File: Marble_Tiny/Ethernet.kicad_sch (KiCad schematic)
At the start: 38 parts, among them J3 BELFUSE_0826-1G1T-43-F, Q1 XTAL_25MHZ_EPSON_TSX-3225_25.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, U7 RTL8211F-CG

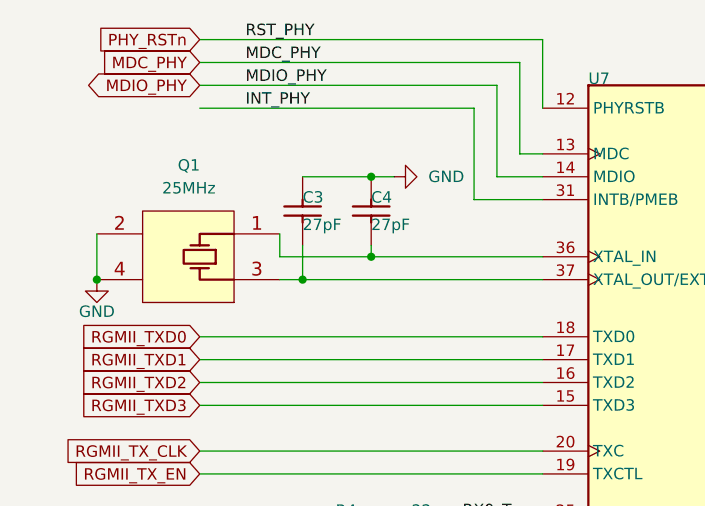
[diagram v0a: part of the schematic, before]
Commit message: components placement and PCB routing
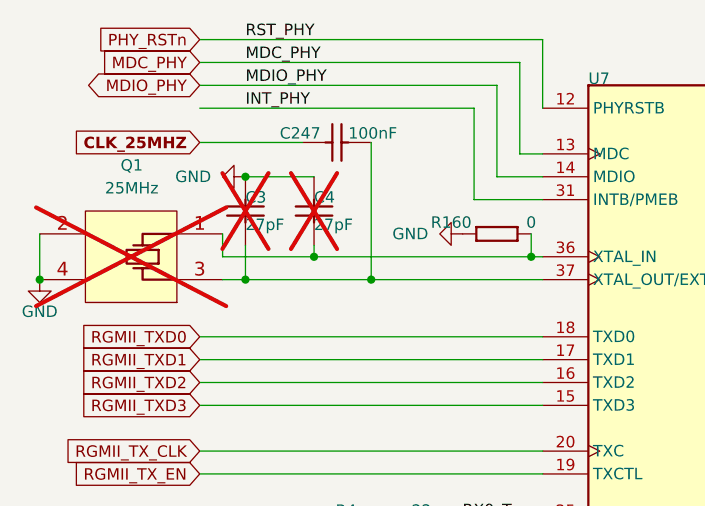
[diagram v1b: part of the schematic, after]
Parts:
- added C247: CC0402_100NF_50V_10%_X7R, Capacitors SMD:CAPC1005X55N, symbol Capacitors SMD:CC0402_100NF_50V_10%_X7R
- added R160: R0402_0R_JUMPER, RESC1005X40N, symbol Resistors_SMD:R0402_0R_JUMPER
- C3, C4, Q1: now not fitted
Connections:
- net GND: now also R160.1
- net at C4.1, Q1.1 (X), U7.36 (XTAL_IN): now also R160.2
- net at C3.1, Q1.3 (X), U7.37 (XTAL_OUT/EXT_CLK): now also C247.1
- new net CLK_25MHZ: C247.2
